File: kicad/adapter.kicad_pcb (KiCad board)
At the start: 16 copper layers, 22 x 31 mm, 2 parts

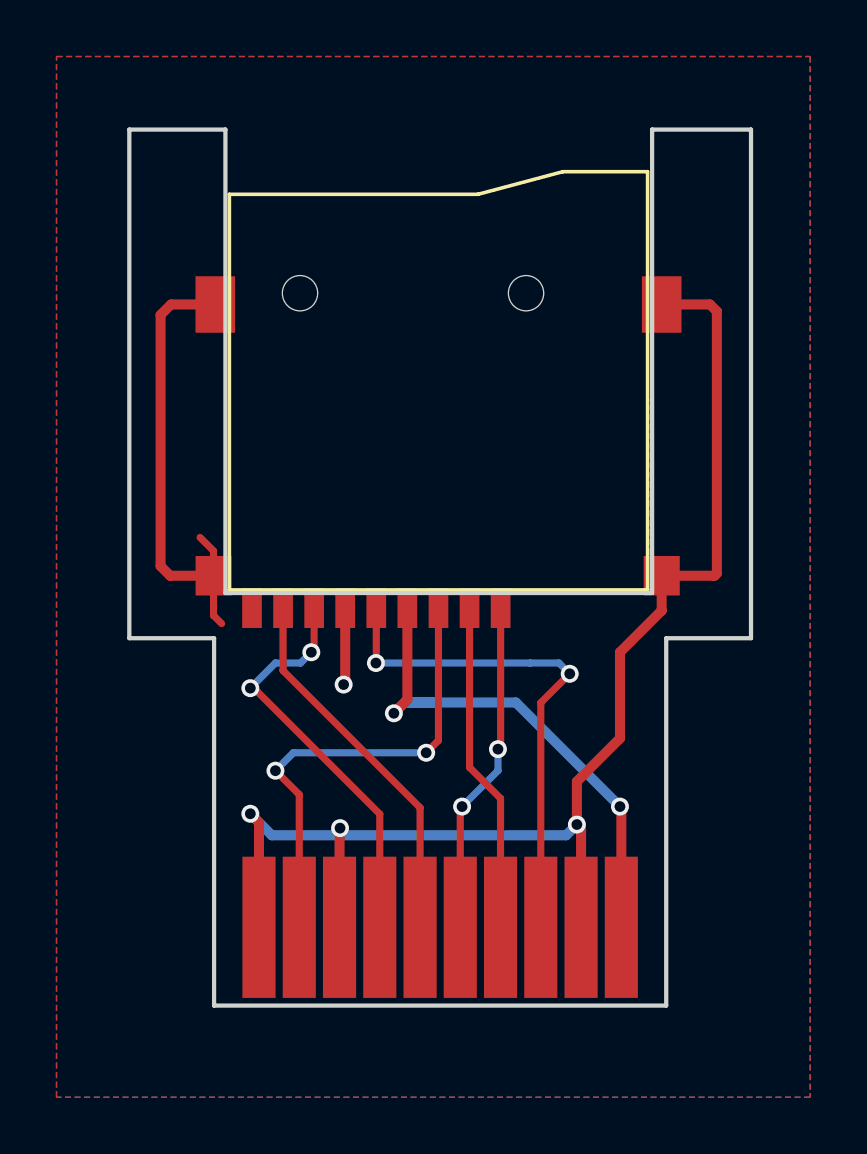
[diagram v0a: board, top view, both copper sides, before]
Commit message: refresh gerbers
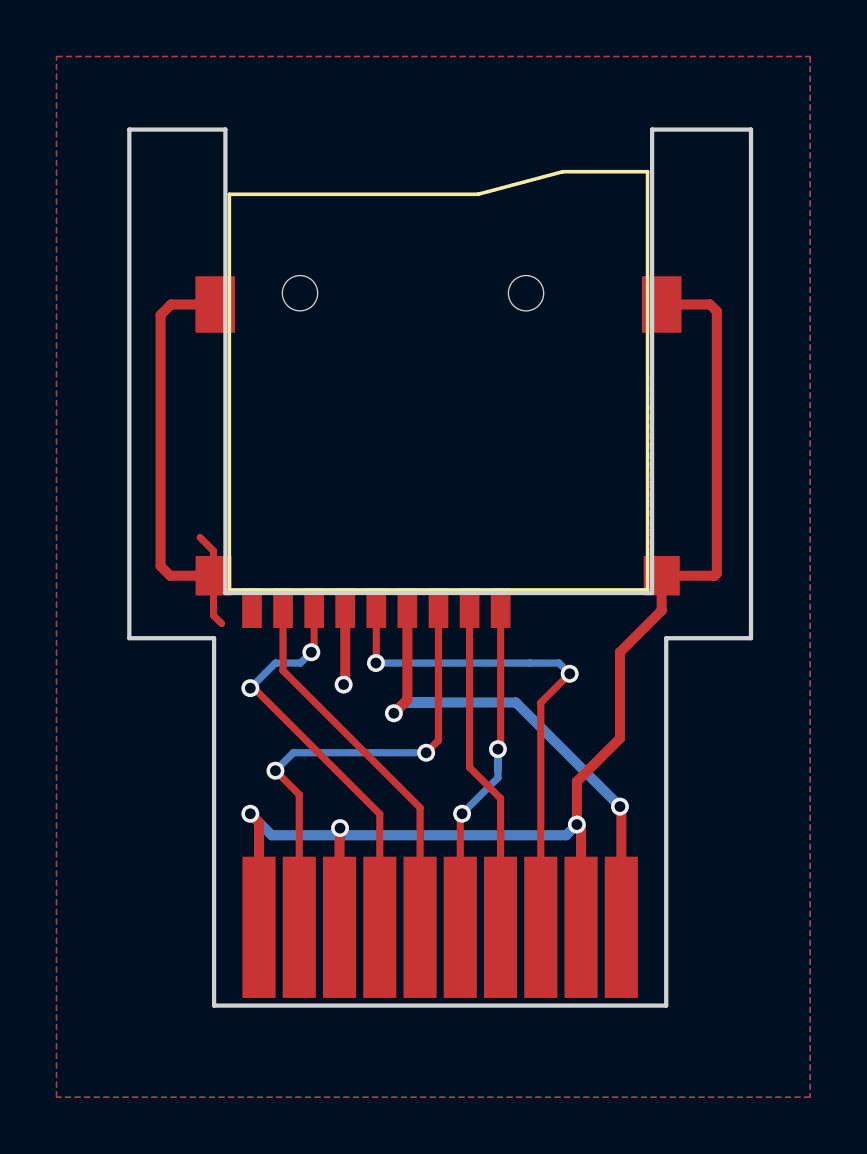
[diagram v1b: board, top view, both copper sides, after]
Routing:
- net /DAT2: track 11.9 -> 12.6 mm
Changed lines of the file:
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@@
     (thickness 1.6)
     (drawings 12)
-    (tracks 89)
+    (tracks 90)
     (zones 0)
     (modules 2)
@@
   (gr_line (start 31.3763 44.3848) (end 46.4763 44.3848) (layer Edge.Cuts) (width 0.15))
   (gr_line (start 46.4763 44.3848) (end 46.4763 27.9848) (layer Edge.Cuts) (width 0.15))
-  (segment (start 35.41522 56.2148) (end 35.41522 52.72278) (width 0.3556) (layer Top) (net 1) (status 400000))
+  (segment (start 35.41522 56.2148) (end 35.41522 52.72278) (width 0.3556) (layer Top) (net 1))
   (via (at 35.433 52.705) (size 0.635) (drill 0.381) (layers Top Bottom) (net 1))
   (segment (start 35.41522 52.72278) (end 35.433 52.705) (width 0.3556) (layer Top) (net 1))
@@
   (segment (start 30.9563 43.7748) (end 30.9563 45.1803) (width 0.254) (layer Top) (net 1) (status 10))
   (segment (start 30.9563 45.1803) (end 31.242 45.466) (width 0.254) (layer Top) (net 1))
-  (segment (start 39.6875 56.2148) (end 39.6875 52.0065) (width 0.254) (layer Top) (net 2))
+  (segment (start 39.6875 56.2148) (end 39.6875 52.2605) (width 0.254) (layer Top) (net 2) (status 400000))
+  (segment (start 41.021 50.927) (end 41.021 49.911) (width 0.254) (layer Bottom) (net 2))
+  (segment (start 39.751 52.197) (end 41.021 50.927) (width 0.254) (layer Bottom) (net 2))
+  (via (at 39.751 52.197) (size 0.635) (drill 0.381) (layers Top Bottom) (net 2))
+  (segment (start 39.6875 52.2605) (end 39.751 52.197) (width 0.254) (layer Top) (net 2))
   (segment (start 41.021 50.673) (end 41.021 49.911) (width 0.254) (layer Bottom) (net 2))
-  (segment (start 39.751 51.943) (end 41.021 50.673) (width 0.254) (layer Bottom) (net 2))
-  (via (at 39.751 51.943) (size 0.635) (drill 0.381) (layers Top Bottom) (net 2))
-  (segment (start 39.6875 52.0065) (end 39.751 51.943) (width 0.254) (layer Top) (net 2))
   (segment (start 41.1163 49.8157) (end 41.1163 44.9248) (width 0.254) (layer Top) (net 2) (status 20))
   (via (at 41.021 49.911) (size 0.635) (drill 0.381) (layers Top Bottom) (net 2))
